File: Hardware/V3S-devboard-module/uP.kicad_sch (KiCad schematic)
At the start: 11 parts, among them U1 V3S, Y1 Crystal_GND23_Small, Y2 Crystal_GND23_Small

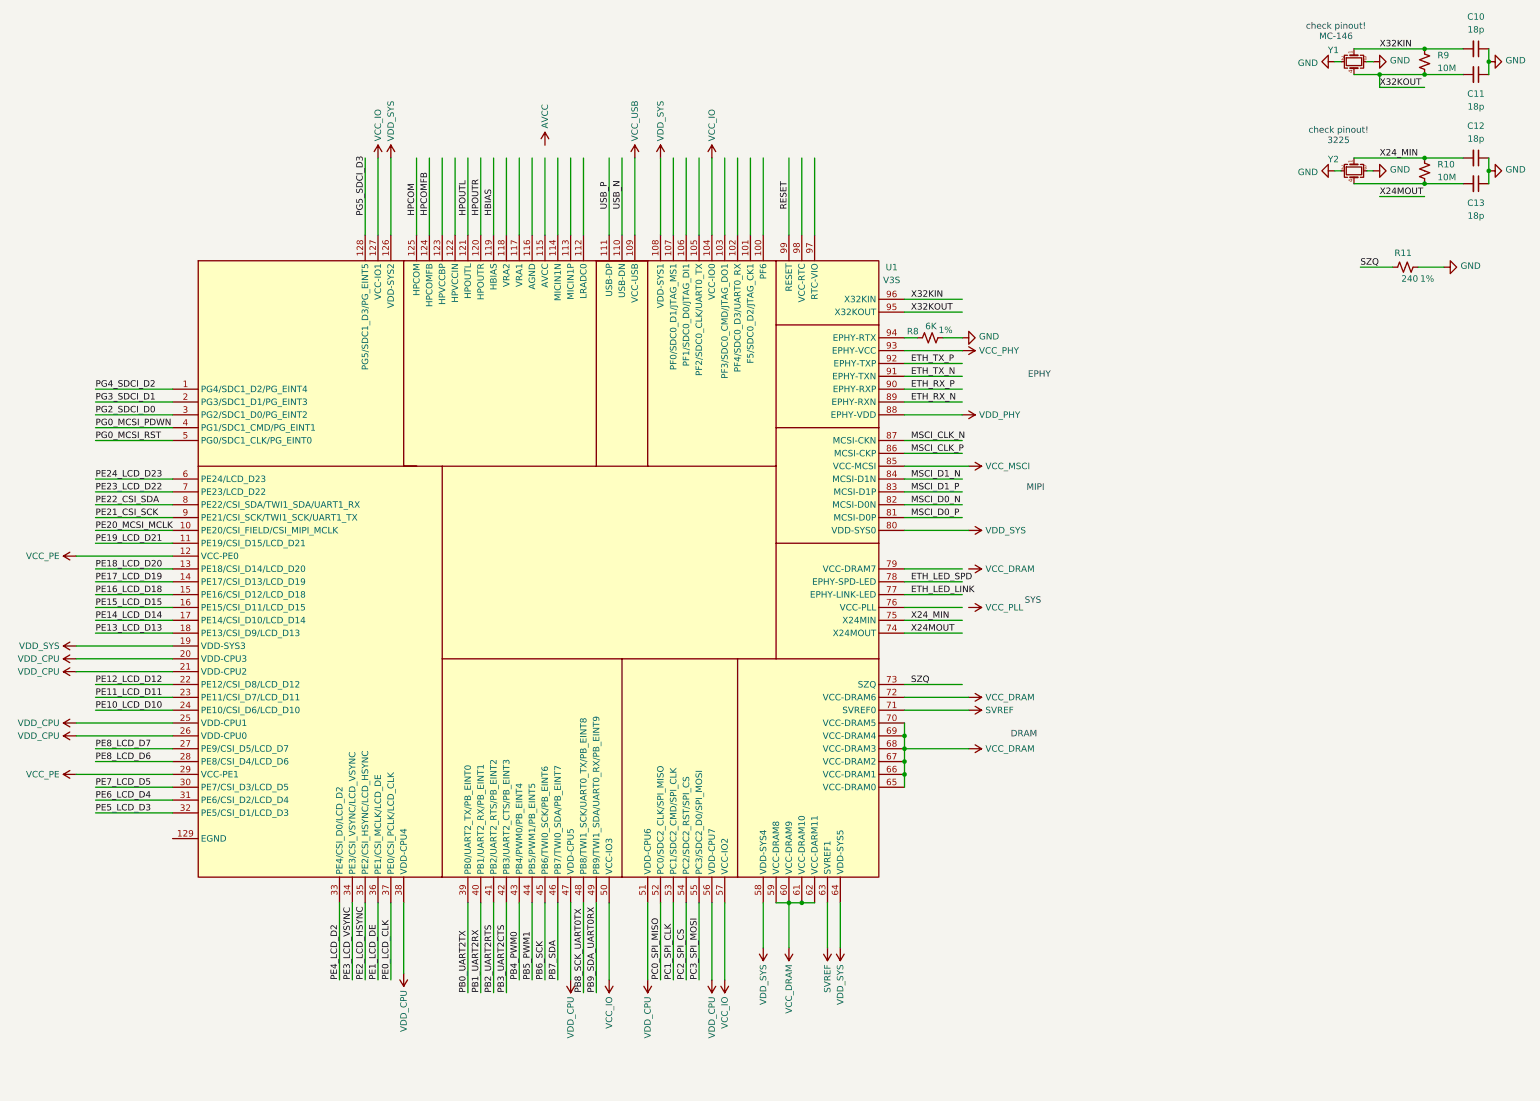
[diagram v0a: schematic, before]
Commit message: more schematic changes
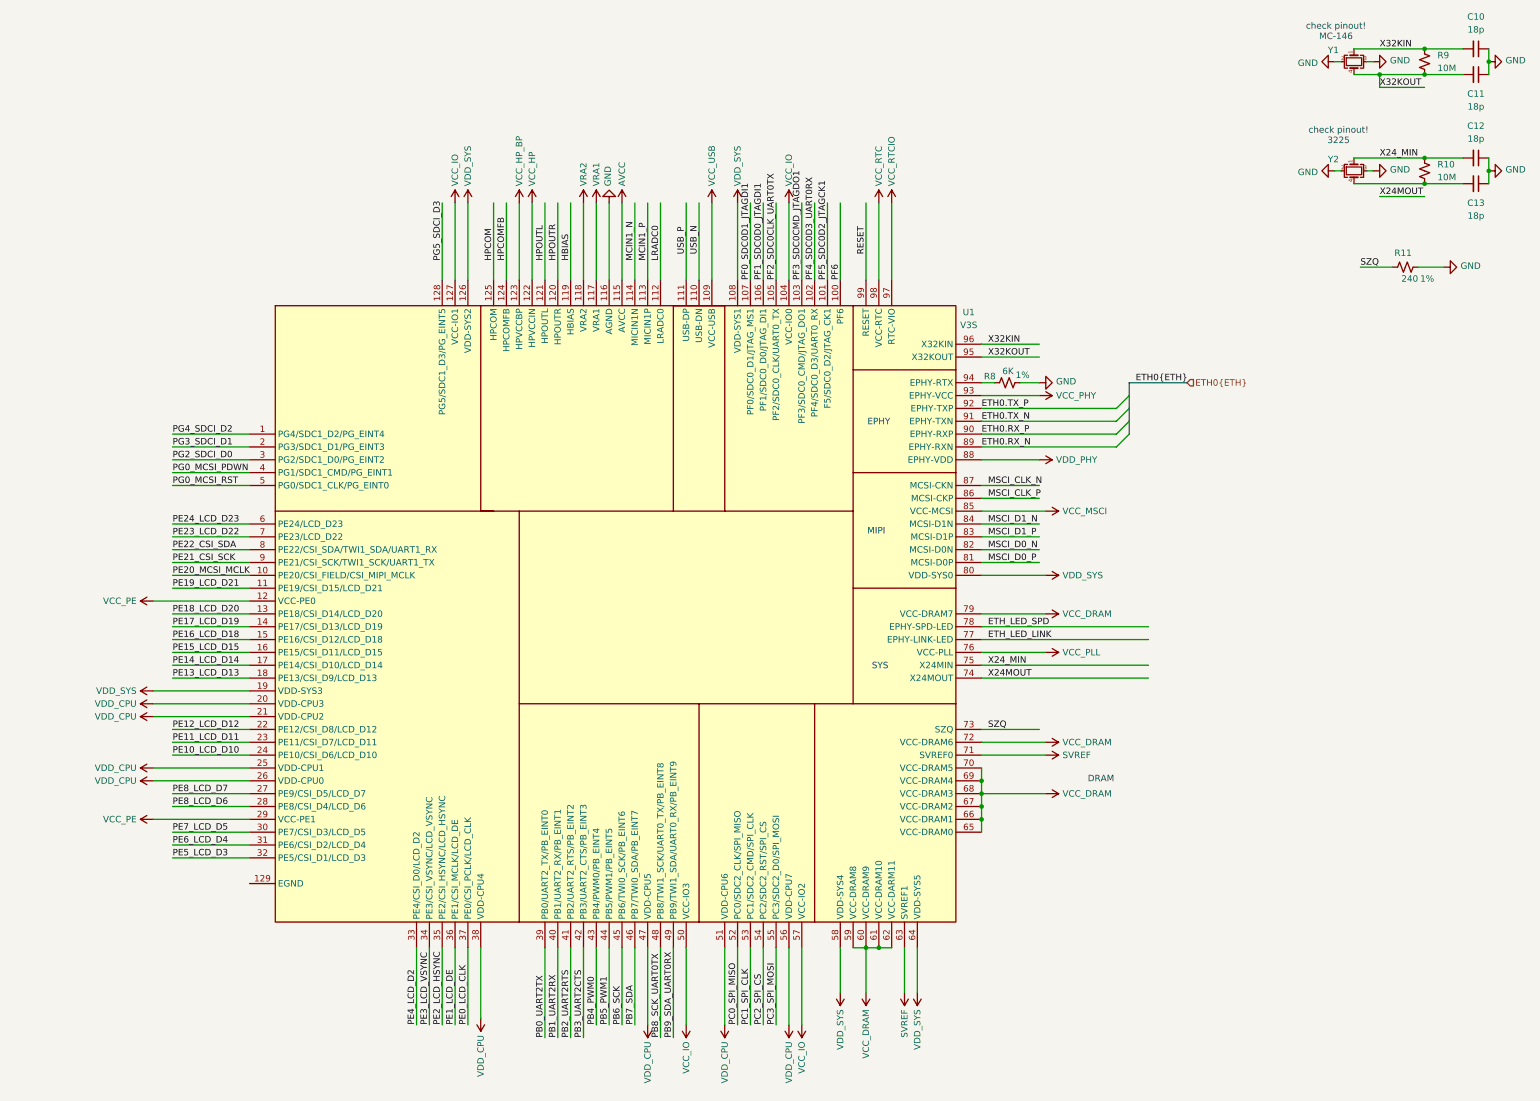
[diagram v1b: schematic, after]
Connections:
- net AVCC: now also U1.115 (AVCC)
- net GND: now also U1.116 (AGND)
- net VCC_DRAM: now also U1.79 (VCC-DRAM7)
- net VCC_PLL: now also U1.76 (VCC-PLL)
- net PF6: now reaches U1.100 (PF6)
- net PF5_SDC0D2_JTAGCK1: now reaches U1.101 (F5/SDC0_D2/JTAG_CK1)
- net PF4_SDC0D3_UART0RX: now reaches U1.102 (PF4/SDC0_D3/UART0_RX)
- net PF3_SDC0CMD_JTAGDO1: now reaches U1.103 (PF3/SDC0_CMD/JTAG_DO1)
- net PF2_SDC0CLK_UART0TX: now reaches U1.105 (PF2/SDC0_CLK/UART0_TX)
- net PF1_SDC0D0_JTAGDI1: now reaches U1.106 (PF1/SDC0_D0/JTAG_DI1)
- net PF0_SDC0D1_JTAGDI1: now reaches U1.107 (PF0/SDC0_D1/JTAG_MS1)
- net LRADC0: now reaches U1.112 (LRADC0)
- net MCIN1_P: now reaches U1.113 (MICIN1P)
- net MCIN1_N: now reaches U1.114 (MICIN1N)
- net VRA1: now reaches U1.117 (VRA1)
- net VRA2: now reaches U1.118 (VRA2)
- net VCC_HP: now reaches U1.122 (HPVCCIN)
- net VCC_HP_BP: now reaches U1.123 (HPVCCBP)
- net VCC_RTCIO: now reaches U1.97 (RTC-VIO)
- net VCC_RTC: now reaches U1.98 (VCC-RTC)
- net ETH_RX_N renamed ETH0.RX_N
- net ETH_RX_P renamed ETH0.RX_P
- net ETH_TX_N renamed ETH0.TX_N
- net ETH_TX_P renamed ETH0.TX_P
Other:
- moved on the sheet: R8, U1
